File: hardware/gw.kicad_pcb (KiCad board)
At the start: 4 copper layers, 47 x 32.9 mm, 21 parts, among them J1 USB_OTG, J2 Conn_01x04, U1 ESP-12F, U2 Ai-Thinker-Ra-02, U3 AMS1117-3.3

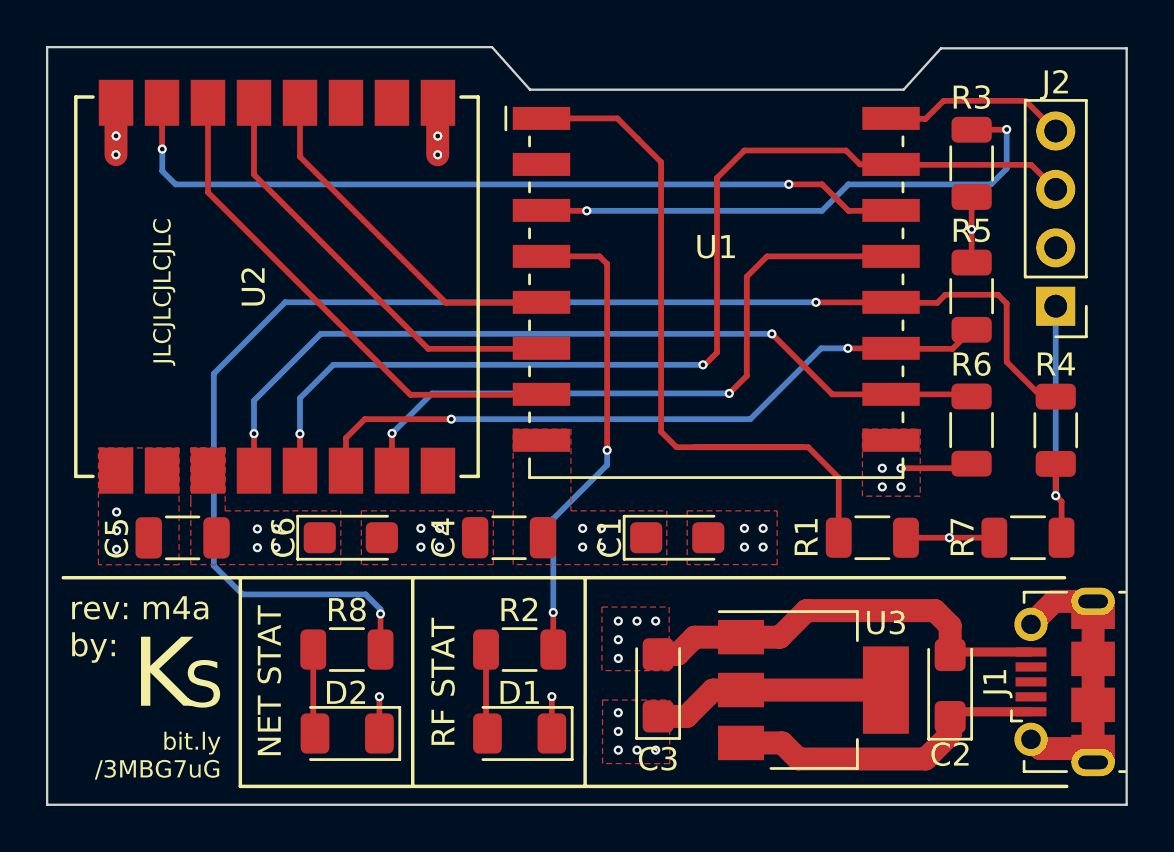
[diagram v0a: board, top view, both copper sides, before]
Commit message: Fix errors
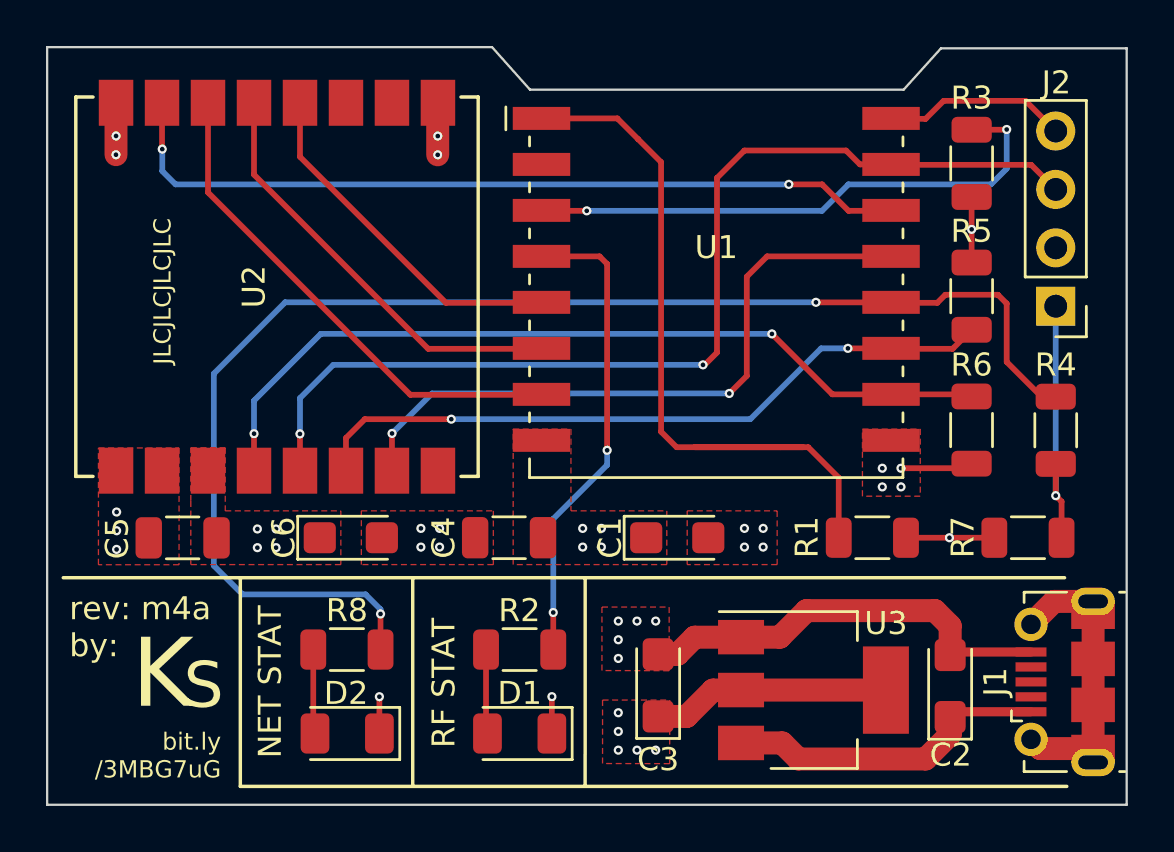
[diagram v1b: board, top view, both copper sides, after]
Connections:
- net /RXD renamed /RXD_D0
